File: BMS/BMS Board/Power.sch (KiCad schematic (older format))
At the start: 18 parts, among them K1 G5PZ-1A_DC12, M21 AO3402, P1 Power_Pad, P2 Power_Pad, P3 Power_Pad, P4 Power_Pad, P5 Power_Pad, P6 Power_Pad, Q1 STD12N60DM2AG

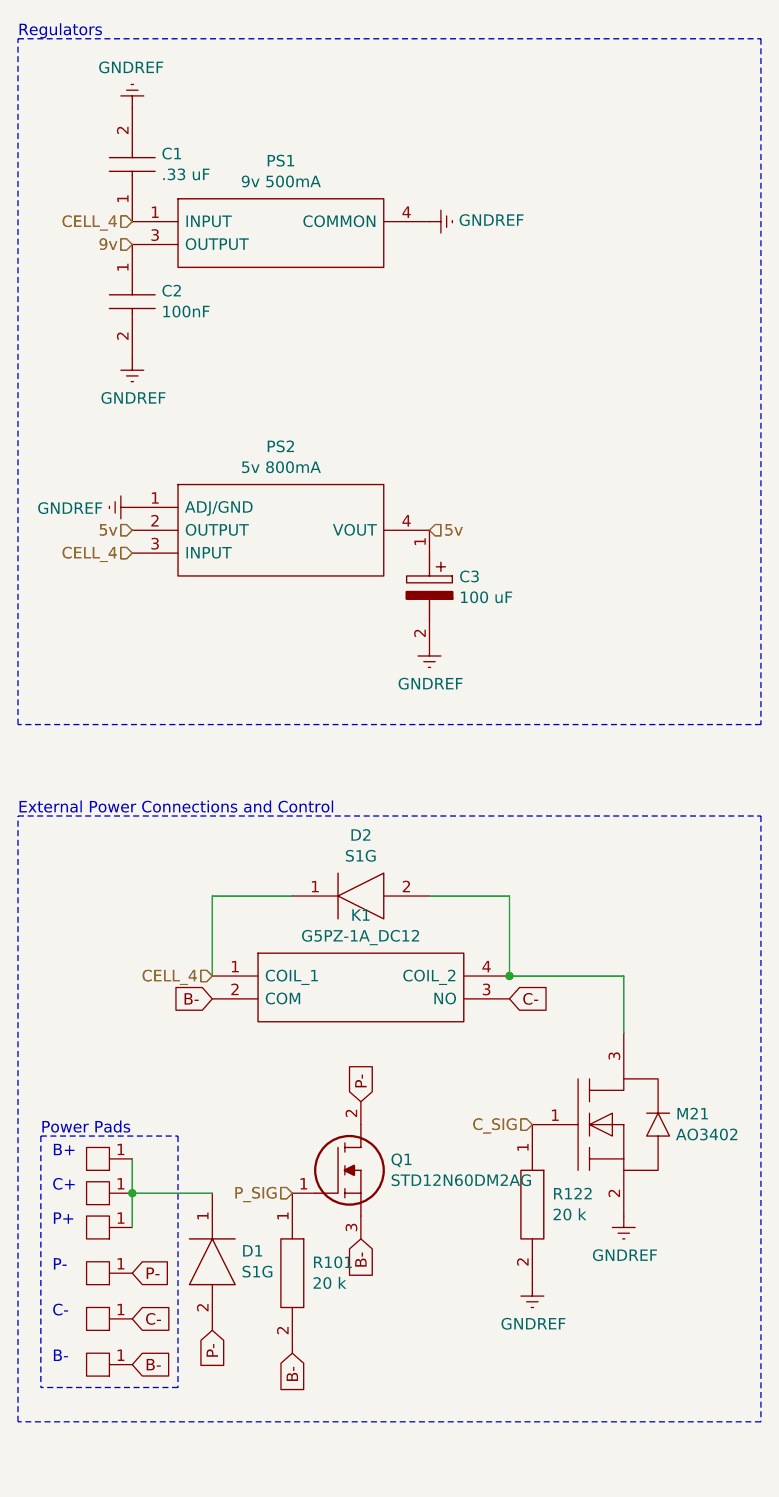
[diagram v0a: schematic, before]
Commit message: ...
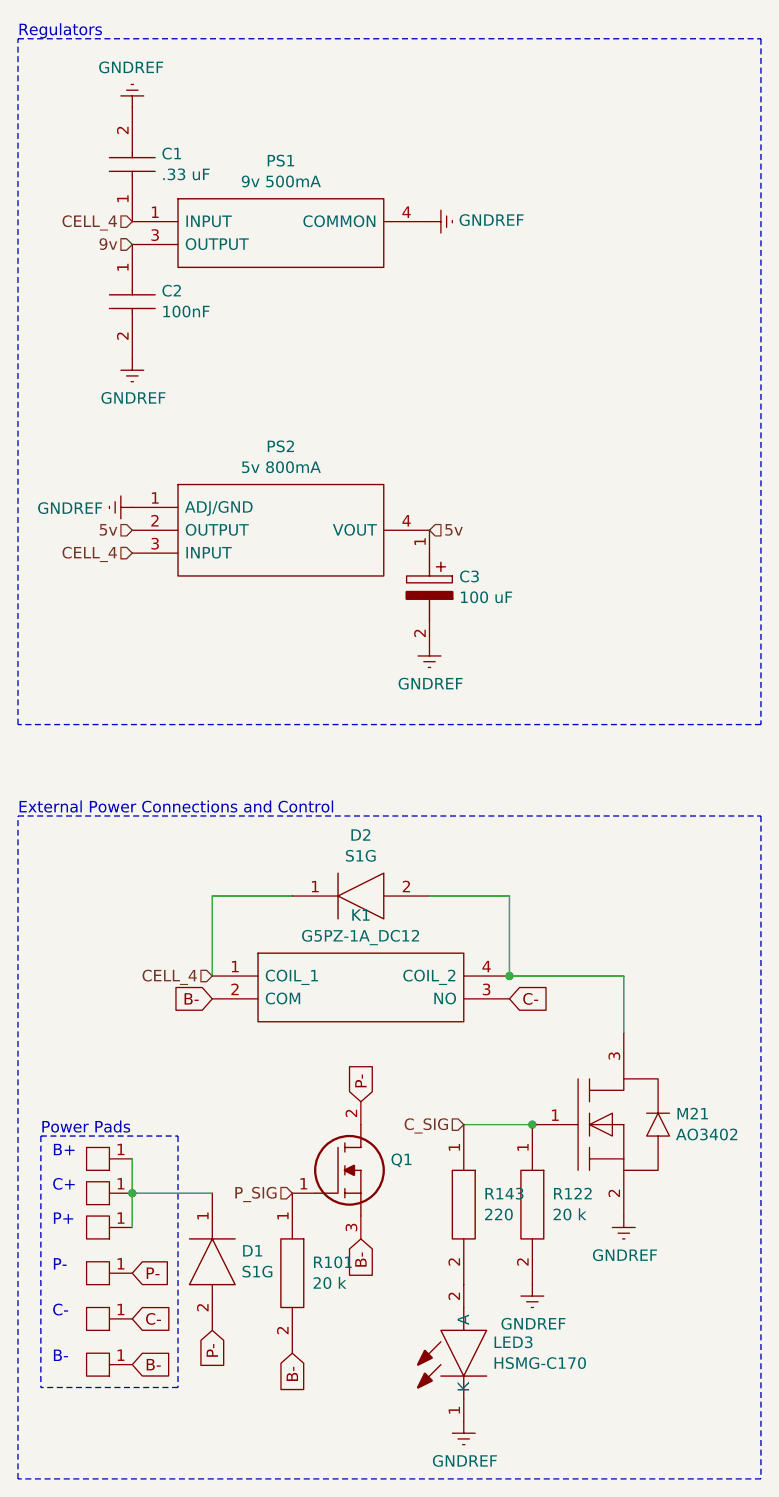
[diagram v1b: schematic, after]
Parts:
- added LED3: HSMG-C170, LEDC2012X80N, symbol SamacSys_Parts:HSMG-C170
- added R143: ERJ-P06F2200V, RESC2012X70N, symbol SamacSys_Parts:ERJ-P06F2200V
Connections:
- net C_SIG: now also R143.1
- net GNDREF: now also LED3.1 (K)
- new net: LED3.2 (A), R143.2
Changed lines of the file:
@@
 P 4000 7700
 F 0 "Q1" H 4180 7746 50  0000 L CNN
-F 1 "STD12N60DM2AG" H 4180 7655 50  0000 L CNN
+F 1 "STD12N60DM2AG" H 4180 7655 50  0001 L CNN
 F 2 "STD13N60DM2" H 3750 7050 50  0001 L CNN
 F 3 "https://www.st.com/resource/en/datasheet/std12n60dm2ag.pdf" H 3750 6950 50  0001 L CNN
@@
 	-1   0    0    1
 $EndComp
-Text HLabel 4800 7500 0    50   Input ~ 0
+Text HLabel 4500 7500 0    50   Input ~ 0
 C_SIG
 Text HLabel 3750 7800 0    50   Input ~ 0
@@
 	2550 6150 5800 6150
 Wire Notes Line
-	5800 8800 2550 8800
+	5800 9050 2550 9050
 Text Notes 2550 6150 0    50   ~ 0
 External Power Connections and Control
@@
 	1    0    0    -1
 $EndComp
-Wire Notes Line
-	2550 8800 2550 6150
-Wire Notes Line
-	5800 6150 5800 8800
 Wire Wire Line
 	3750 6500 3400 6500
@@
 Text GLabel 3400 8400 3    50   Input ~ 0
 P-
+$Comp
+L SamacSys_Parts:ERJ-P06F2200V R143
+U 1 1 5EF455EC
+P 4500 7850
+F 0 "R143" V 4454 7938 50  0000 L CNN
+F 1 "ERJ-P06F2200V" H 4350 7600 50  0001 L CNN
+F 2 "RESC2012X70N" H 4350 7500 50  0001 L CNN
+F 3 "https://componentsearchengine.com/Datasheets/1/ERJ-P06F2200V.pdf" H 4700 7800 50  0001 L CNN
+F 4 "Thick Film Resistors - SMD 0805 220ohms 0.5W 1% AEC-Q200" H 4350 7400 50  0001 L CNN "Description"
+F 5 "0.7" H 4350 7300 50  0001 L CNN "Height"
+F 6 "667-ERJ-P06F2200V" H 4350 7200 50  0001 L CNN "Mouser Part Number"
+F 7 "https://www.mouser.com/Search/Refine.aspx?Keyword=667-ERJ-P06F2200V" H 4350 7100 50  0001 L CNN "Mouser Price/Stock"
+F 8 "Panasonic" H 4350 7000 50  0001 L CNN "Manufacturer_Name"
+F 9 "ERJ-P06F2200V" H 4350 6900 50  0001 L CNN "Manufacturer_Part_Number"
+F 10 "220" V 4545 7938 50  0000 L CNN "Resistance"
+	1    4500 7850
+	0    1    1    0
+$EndComp
+$Comp
+L SamacSys_Parts:HSMG-C170 LED3
+U 1 1 5EF477B4
+P 4500 8450
+F 0 "LED3" V 4496 8322 50  0000 R CNN
+F 1 "HSMG-C170" V 4405 8322 50  0000 R CNN
+F 2 "LEDC2012X80N" H 4250 8050 50  0001 L BNN
+F 3 "" H 4650 8500 50  0001 L BNN
+F 4 "Green LED, 15 mcd 170 , 2-pin 0805 SMD Package" H 4250 7950 50  0001 L BNN "Description"
+F 5 "0.8" H 4250 7850 50  0001 L BNN "Height"
+F 6 "630-HSMG-C170" H 4250 7750 50  0001 L BNN "Mouser Part Number"
+F 7 "https://www.mouser.co.uk/ProductDetail/Broadcom-Avago/HSMG-C170?qs=YDL0qNrpDT4lm8ArMPkMEA%3D%3D" H 4250 7650 50  0001 L BNN "Mouser Price/Stock"
+F 8 "Avago Technologies" H 4250 7550 50  0001 L BNN "Manufacturer_Name"
+F 9 "HSMG-C170" H 4250 7450 50  0001 L BNN "Manufacturer_Part_Number"
+	1    4500 8450
+	0    -1   -1   0
+$EndComp
+$Comp
+L power:GNDREF #PWR0155
+U 1 1 5EF48294
+P 4500 8800
+F 0 "#PWR0155" H 4500 8550 50  0001 C CNN
+F 1 "GNDREF" H 4505 8627 50  0000 C CNN
+F 2 "" H 4500 8800 50  0001 C CNN
+F 3 "" H 4500 8800 50  0001 C CNN
+	1    4500 8800
+	1    0    0    -1
+$EndComp
+Wire Notes Line
+	2550 9050 2550 6150
+Wire Notes Line
+	5800 6150 5800 9050
+Wire Wire Line
+	4500 7500 4800 7500
+Connection ~ 4800 7500
 $EndSCHEMATC
